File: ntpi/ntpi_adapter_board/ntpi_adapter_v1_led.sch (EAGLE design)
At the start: 7 parts, among them Q1 BC849C

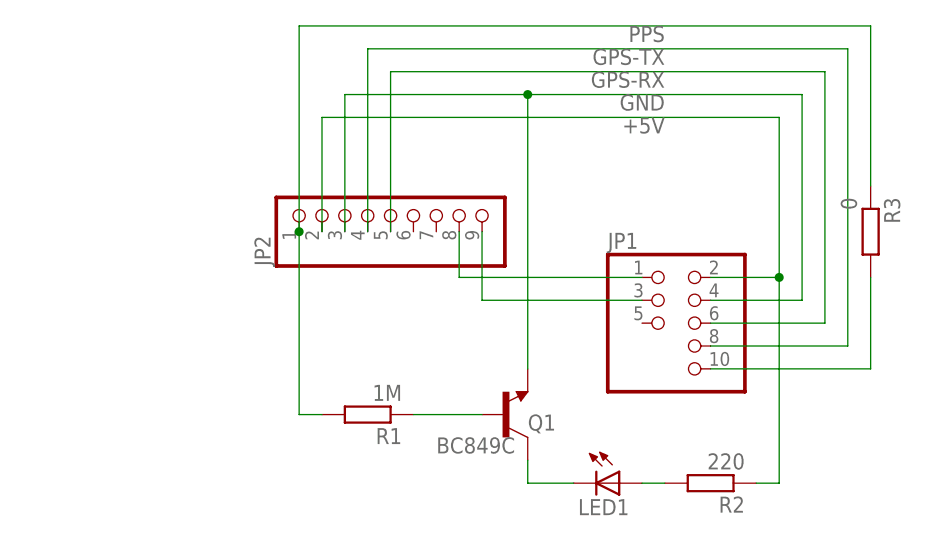
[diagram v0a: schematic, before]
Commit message: NTPi adapter board v1.1
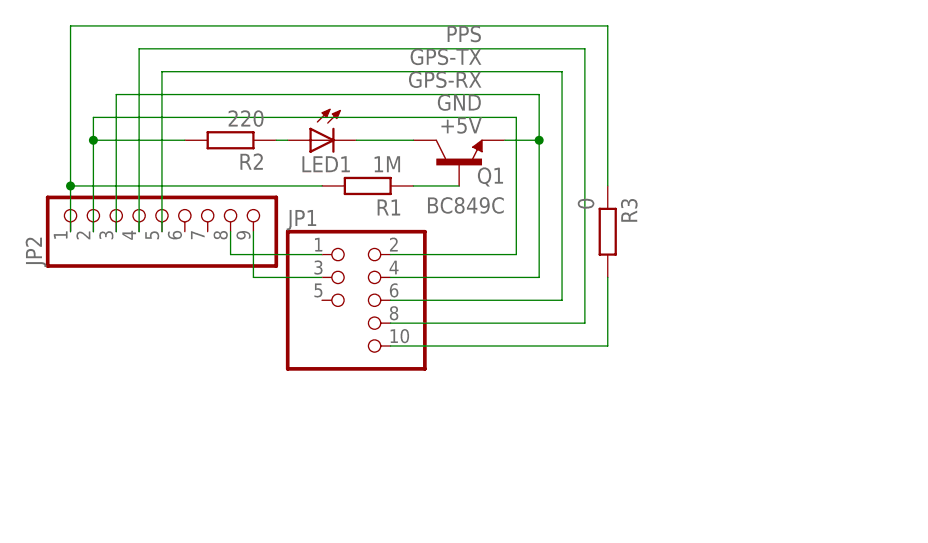
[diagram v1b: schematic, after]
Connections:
- removed net N$9: LED1.A, R2.2
- new net N$2: LED1.A, R2.1
- net +5V: now also R2.2; no longer R2.1
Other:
- moved on the sheet: JP1, JP2, LED1, Q1, R1, R2, R3
